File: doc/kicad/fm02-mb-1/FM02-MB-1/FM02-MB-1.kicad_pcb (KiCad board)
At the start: 2 copper layers, 28 x 28 mm, 16 parts, among them J1 Conn_01x04, J2 Conn_01x06, Q1 Q_NMOS_DGS, Q2 Q_NMOS_DGS, Q3 Q_NMOS_DGS, Q4 Q_NMOS_DGS, U1 MPU-6050

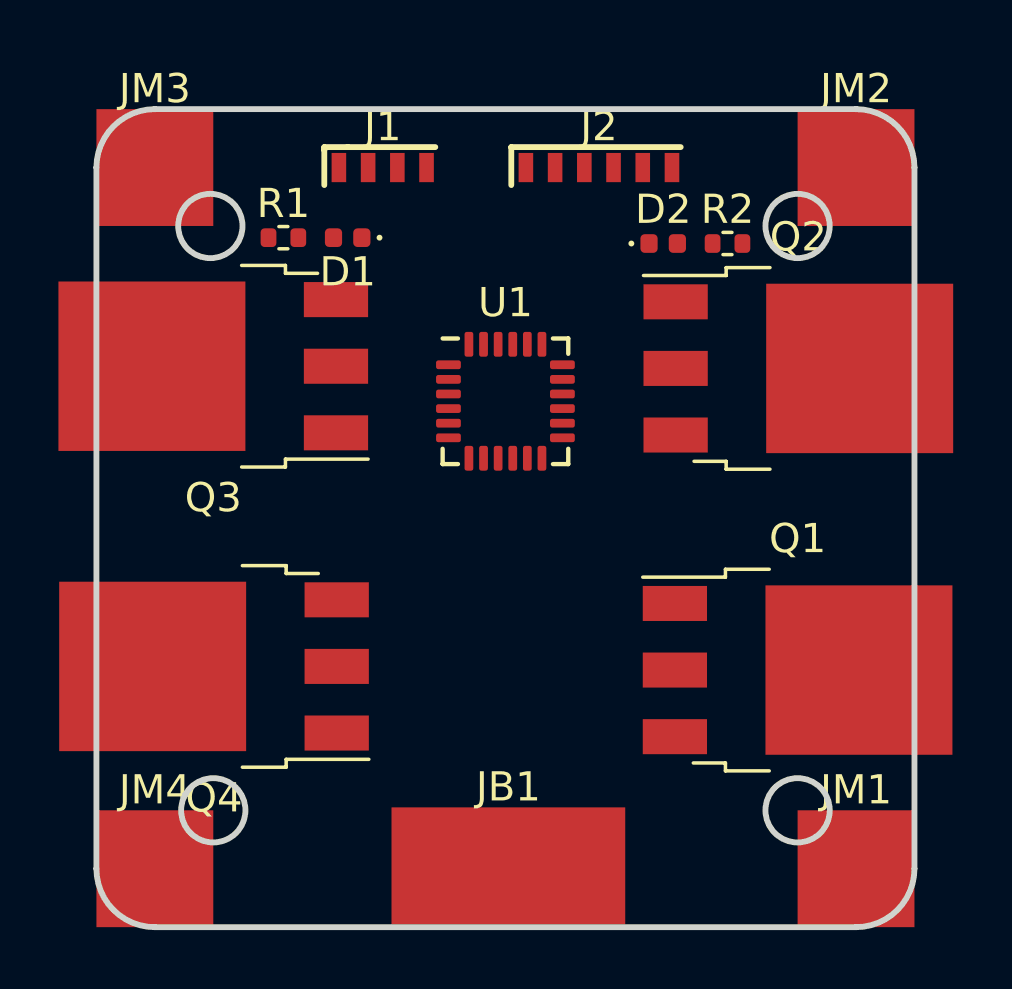
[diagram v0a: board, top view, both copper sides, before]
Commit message: doc/kicad: FM02-MB-1 v0.1
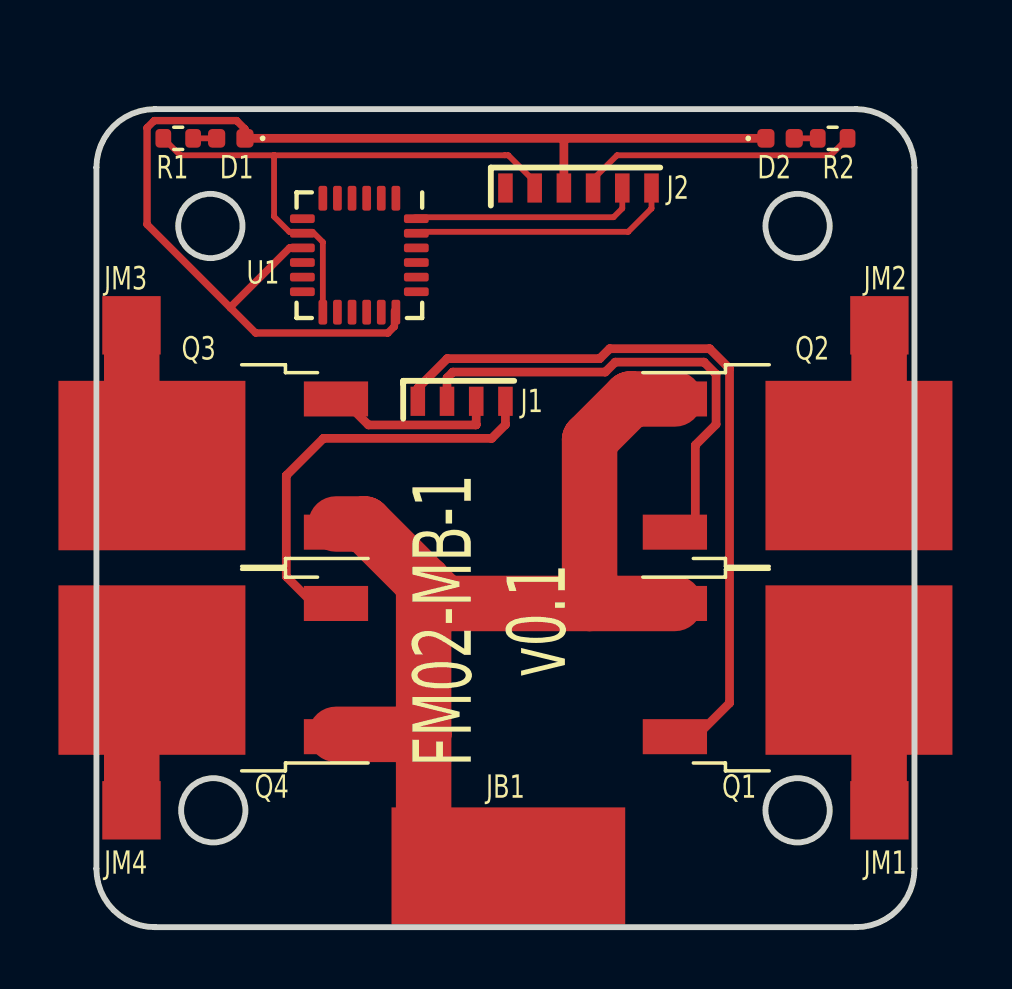
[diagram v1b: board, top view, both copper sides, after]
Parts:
- JM1, JM2, JM3, JM4: footprint Connector_SMD:CSMD-JM1P -> Connector_SMD:CSMD-JM2
- Q1, Q2, Q3, Q4: value Q_NMOS_DGS -> Q_NMOS_DSG; footprint Package_TO_SOT_SMD:TO-252-3_TabPin2 -> Package_TO_SOT_SMD:TO-252-2
- moved J1 8.44 mm to (152.5, 80.0)
- moved U1 7.07 mm to (149.0, 75.0), turned to 270 degrees
- moved JM2 5.46 mm to (166.8, 77.4)
- moved JM3 5.46 mm to (141.2, 77.4)
- moved D2 5.38 mm to (163.4, 71.0)
- moved D1 5.25 mm to (144.6, 71.0)
- moved R2 5.09 mm to (165.2, 71.0), turned to 180 degrees
- moved R1 4.95 mm to (142.8, 71.0)
- moved Q3 3.40 mm to (144.0, 82.2)
- moved Q2 3.33 mm to (164.0, 82.2)
- moved JM1 2.15 mm to (166.8, 94.0)
- moved JM4 2.15 mm to (141.2, 94.0)
- moved J2 0.99 mm to (156.5, 72.7)
- moved Q4 0.13 mm to (144.0, 89.2)
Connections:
- J2 pad 5: /SCL1 -> /SDA1
- J2 pad 6: /SDA1 -> /SCL1
- Q1 pad 2: /QC1 -> /M1
- Q1 pad 3: /M1 -> /QC1
- Q2 pad 2: /QC2 -> /M2
- Q2 pad 3: /M2 -> /QC2
- Q3 pad 2: /QC3 -> /M3
- Q3 pad 3: /M3 -> /QC3
- Q4 pad 2: /QC4 -> /M4
- Q4 pad 3: /M4 -> /QC4
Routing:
- net GND: track 0.00 -> 40.8 mm
- net +BATT: track 0.00 -> 39.1 mm
- net /QC1: track 0.00 -> 25.1 mm
- net +3V3: track 0.00 -> 19.9 mm
- net /QC2: track 0.00 -> 16.1 mm
- net /QC4: track 0.00 -> 13.9 mm
- net /LED2: track 0.00 -> 9.29 mm
- net /SCL1: track 0.00 -> 8.93 mm
- net /SDA1: track 0.00 -> 7.92 mm
- net /QC3: track 0.00 -> 5.64 mm
- net /M2: track 0.00 -> 4.89 mm
- net /M4: track 0.00 -> 4.89 mm
- net /M1: track 0.00 -> 4.89 mm
- net /M3: track 0.00 -> 4.69 mm
- net Net-(D2-Pad2): track 0.00 -> 0.92 mm
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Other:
- board text added: "FM02-MB-1 v0.1"
